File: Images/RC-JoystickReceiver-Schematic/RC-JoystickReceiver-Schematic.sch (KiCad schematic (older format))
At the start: 3 parts

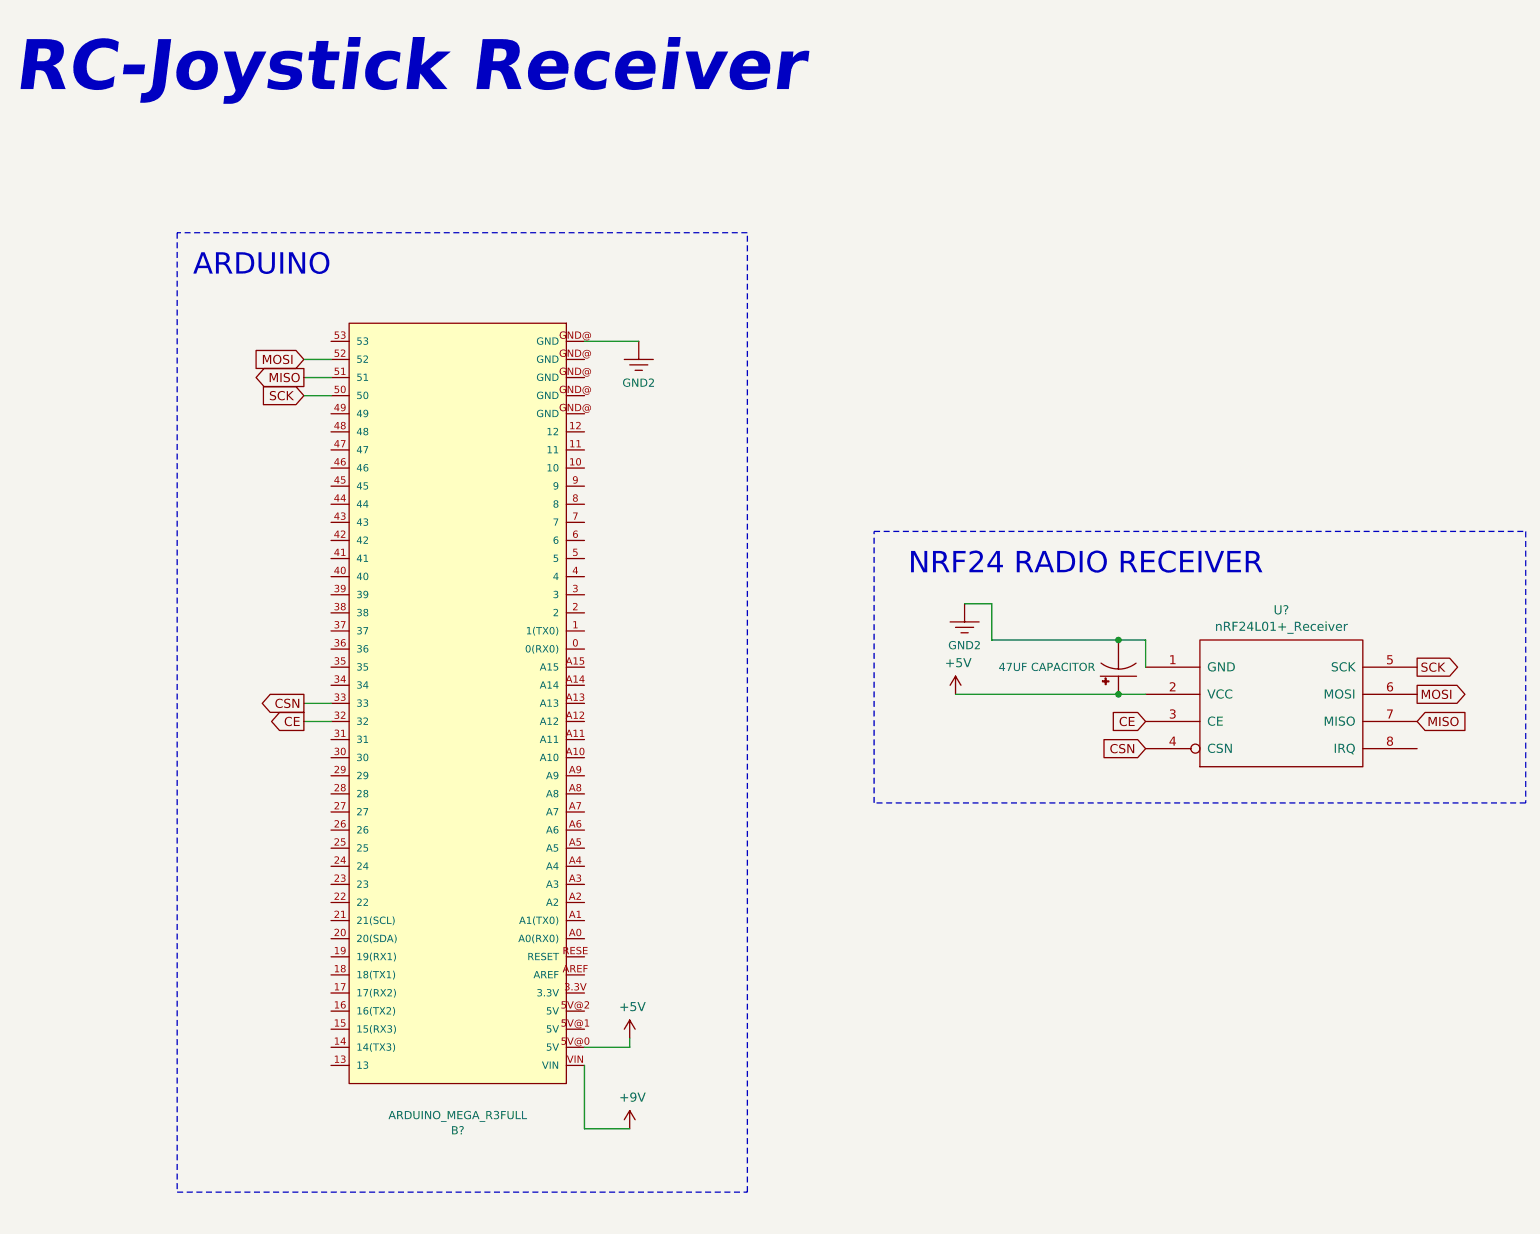
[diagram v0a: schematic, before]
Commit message: Update schematic
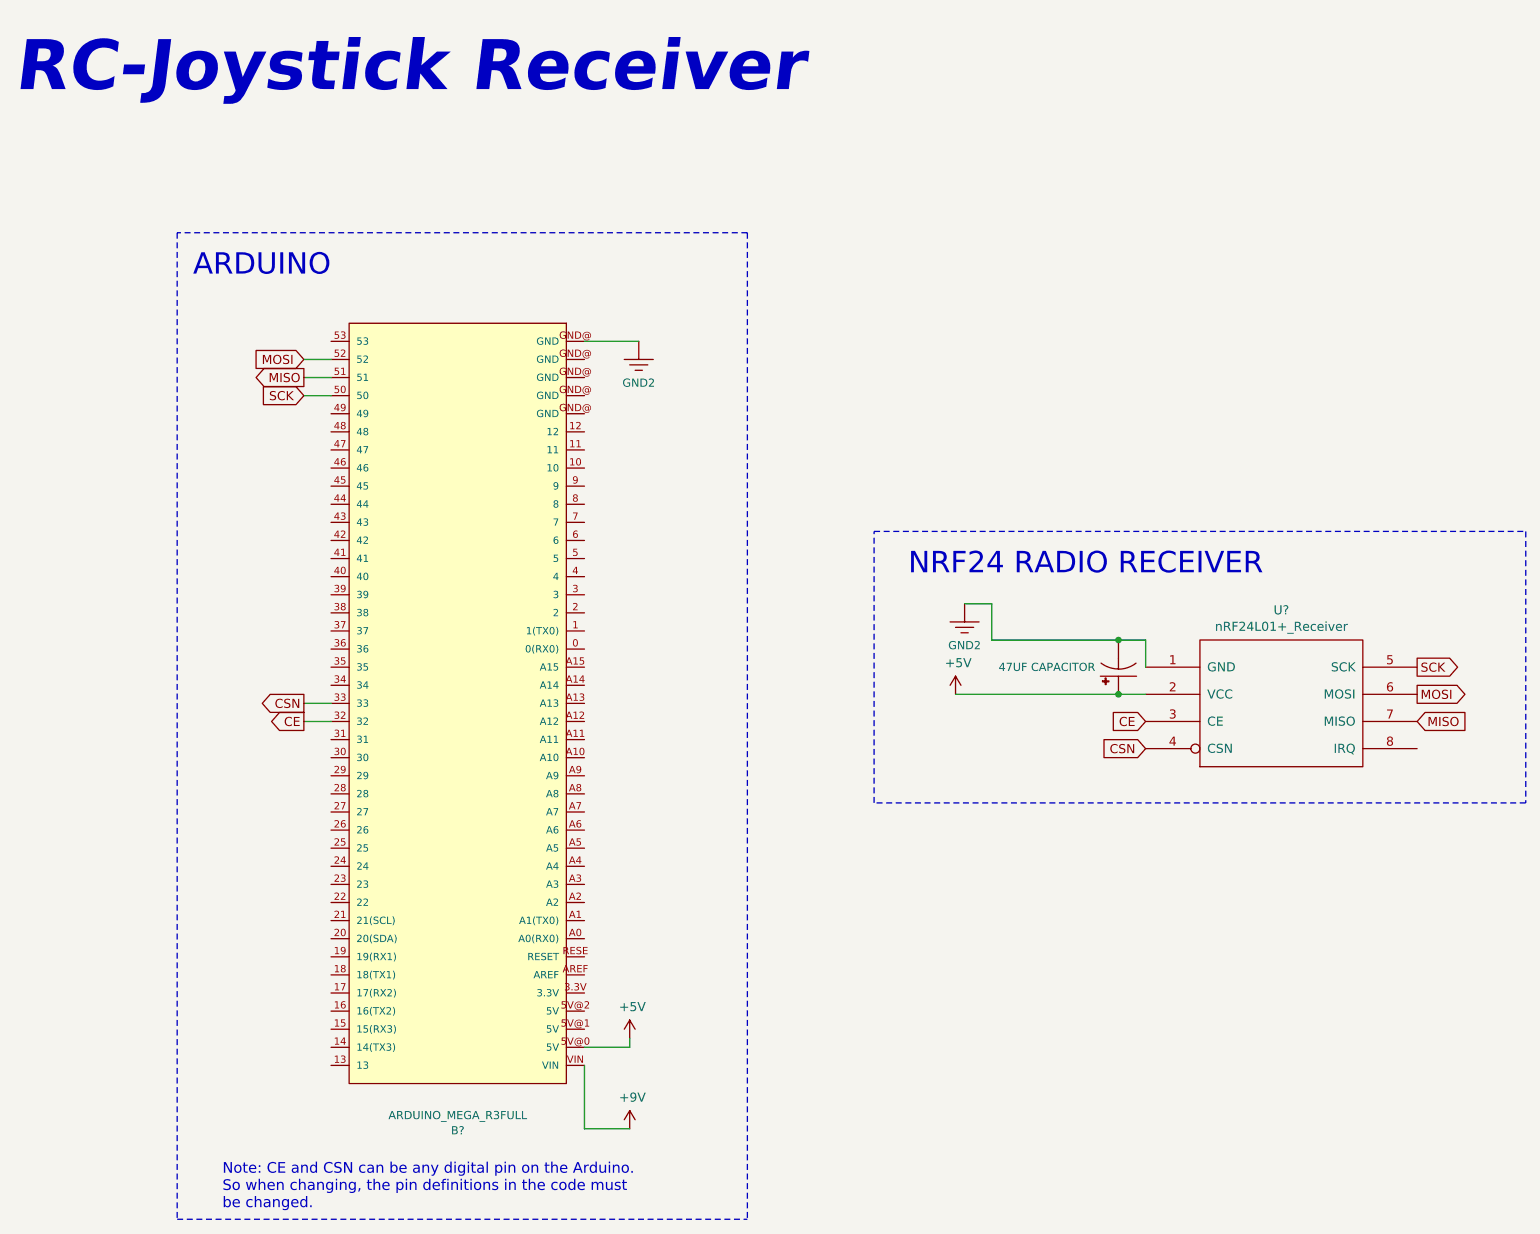
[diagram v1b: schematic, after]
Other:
- note added: "Note: CE and CSN can be any digital pin on the Arduino. \nSo when changing, the pin definitions in the code must \nbe changed."
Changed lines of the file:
@@
 	3950 6900 4200 6900
 Wire Notes Line
-	1700 7250 4850 7250
-Wire Notes Line
-	4850 7250 4850 1950
+	1700 7400 4850 7400
 Wire Notes Line
 	4850 1950 1700 1950
-Wire Notes Line
-	1700 1950 1700 7250
 Wire Notes Line
 	9150 3600 9150 5100
@@
 Wire Wire Line
 	6000 4500 6900 4500
+Text Notes 1950 7350 0    59   ~ 0
+Note: CE and CSN can be any digital pin on the Arduino. \nSo when changing, the pin definitions in the code must \nbe changed.
+Wire Notes Line
+	4850 1950 4850 7400
+Wire Notes Line
+	1700 1950 1700 7400
 $EndSCHEMATC
